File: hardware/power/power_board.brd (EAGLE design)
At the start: 75 x 64.5 mm, 6 parts, among them J1 FASTON_MALE_RA_BLADE, J2 FASTON_MALE_RA_BLADE, J3 12v, J4 5v, U1 PDQ30-Q24-S5-D, U2 PDQ30-Q24-S12-D

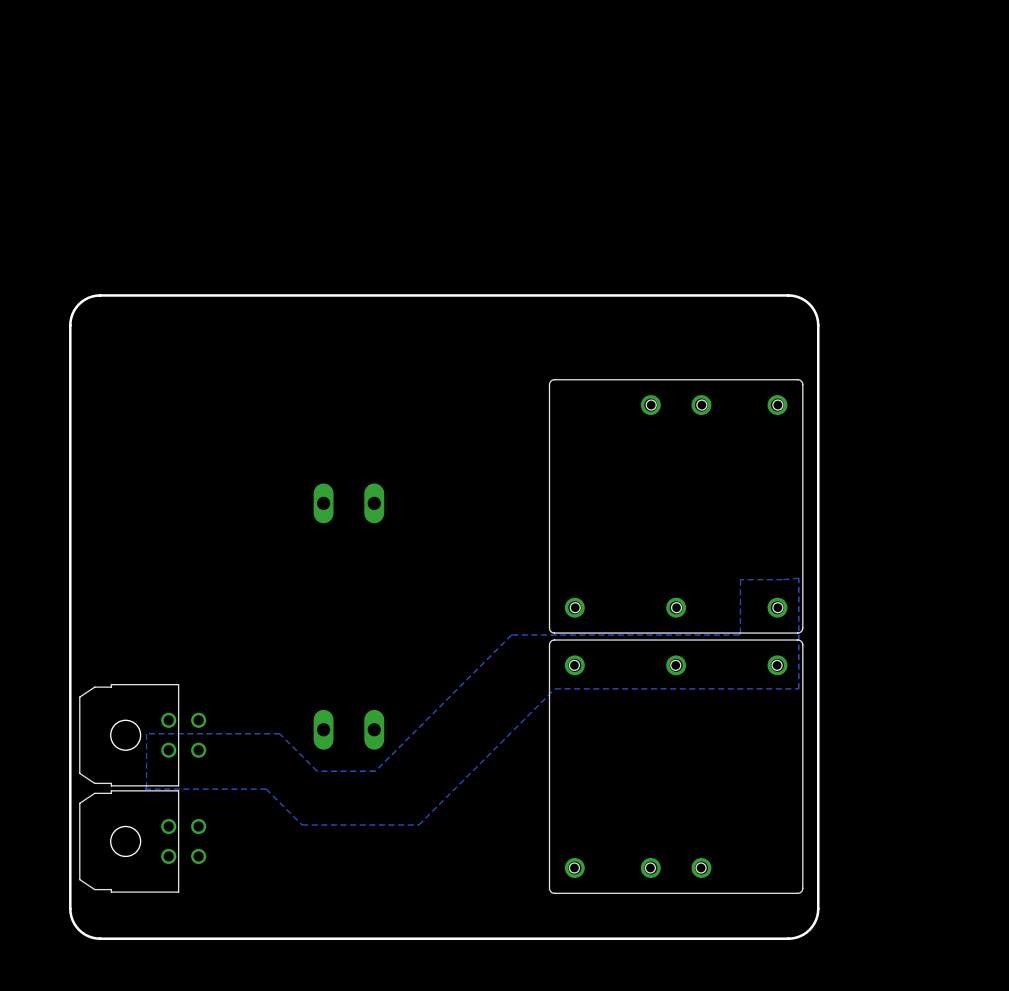
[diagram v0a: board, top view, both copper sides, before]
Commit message: Power updates
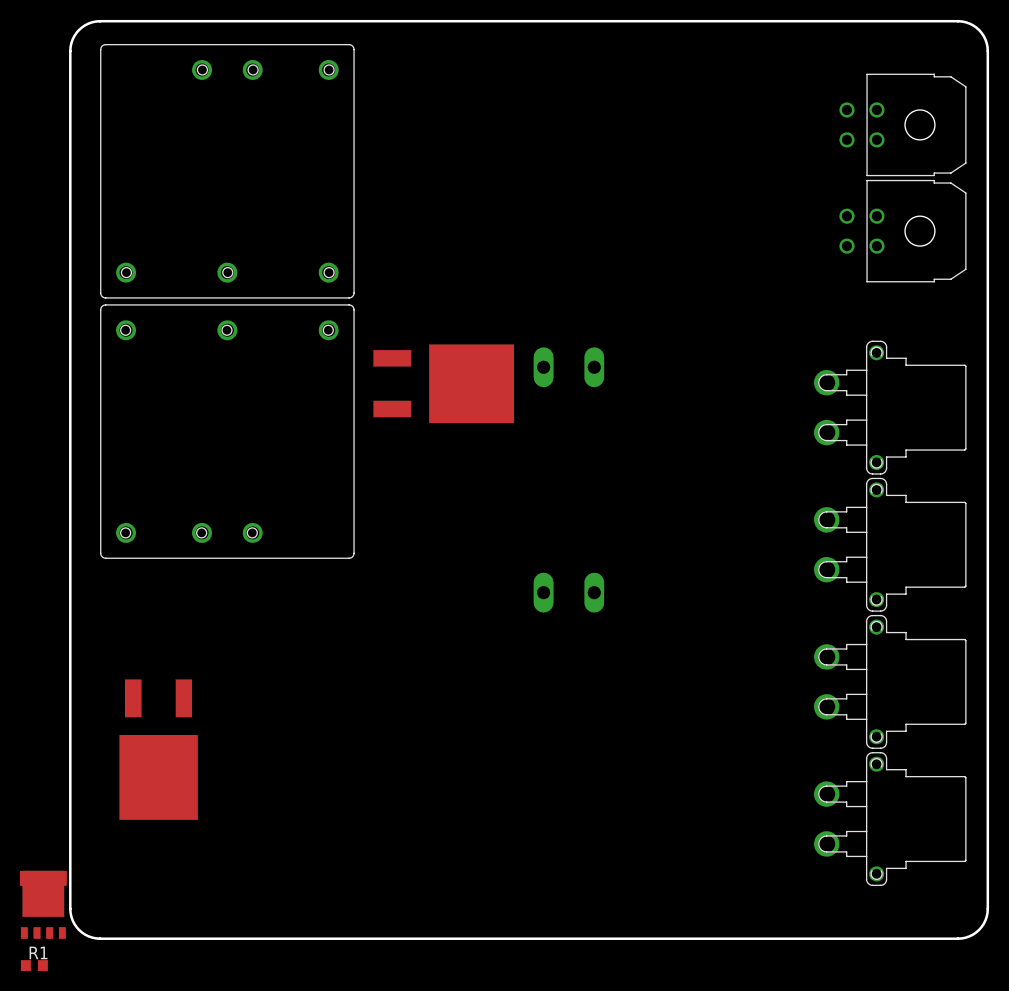
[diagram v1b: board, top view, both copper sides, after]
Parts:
- added J5, J6, J7, J8: XT30PW-F, timlib:XT30PW-F
- added R1: 100, rcl:R0603
- added U$10, U$9: 2, timlib:PWR163
- added U$11: PSMN1R0-40YSH, timlib:LFPAK56E
- moved J3 107.3 mm to (85.2, 81.6), turned to 90 degrees
- moved J4 94.3 mm to (85.2, 71.0), turned to 90 degrees
- moved U2 74.8 mm to (15.8, 77.0), turned to 0 degrees
- moved U1 45.6 mm to (15.8, 50.9), turned to 180 degrees
- moved J1 42.5 mm to (50.0, 57.3), turned to 180 degrees
- moved J2 23.8 mm to (50.0, 34.7), turned to 180 degrees
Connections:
- new net N$1: U$10.P$1, U$11.5
- net +24V: now also J5.P$2, J6.P$2, J7.P$2, J8.P$2
- net GND: now also J5.P$1, J6.P$1, J7.P$1, J8.P$1, U$11.1, U$11.2, U$11.3
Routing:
- removed copper zone on layer 16, net GND_5V
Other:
- board size 75 x 64.5 mm -> 92 x 92 mm
